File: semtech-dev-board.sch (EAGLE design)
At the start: 62 parts, among them Q1 BSS123, Q2 32MHz, U1 SEMTECH_SX1236, U2 QUALCOMM-TDK_B3588, U3 MIC5219 3.3V, U4 QUALCOMM-TDK_B3710

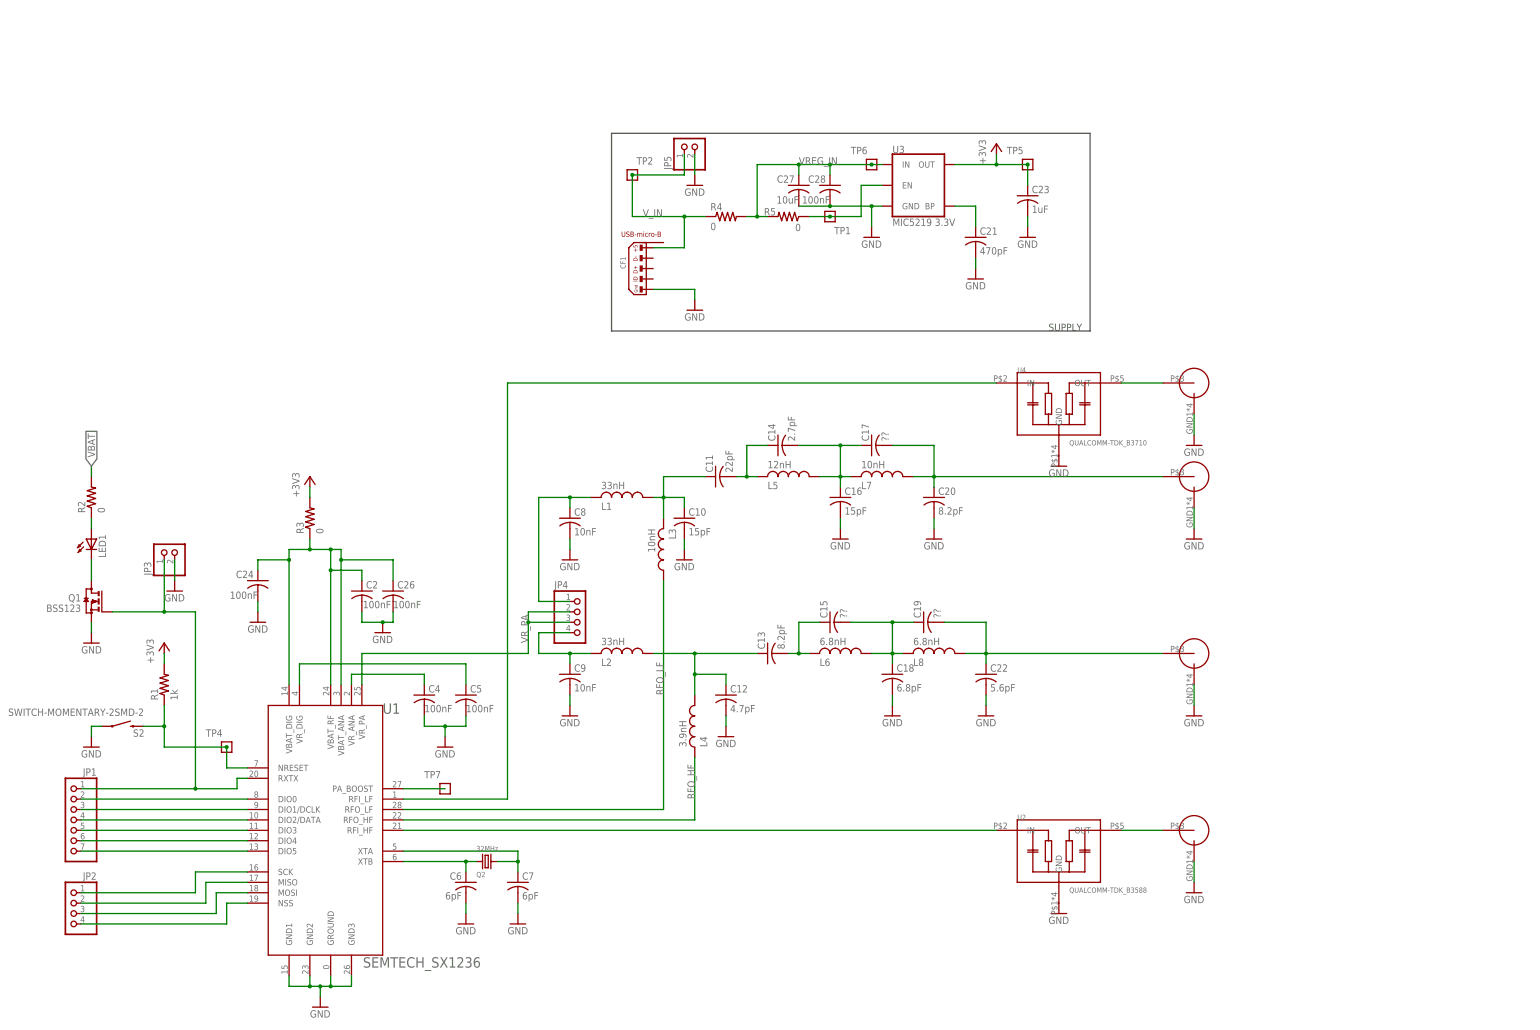
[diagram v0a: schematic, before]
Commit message: Tuesday D/R
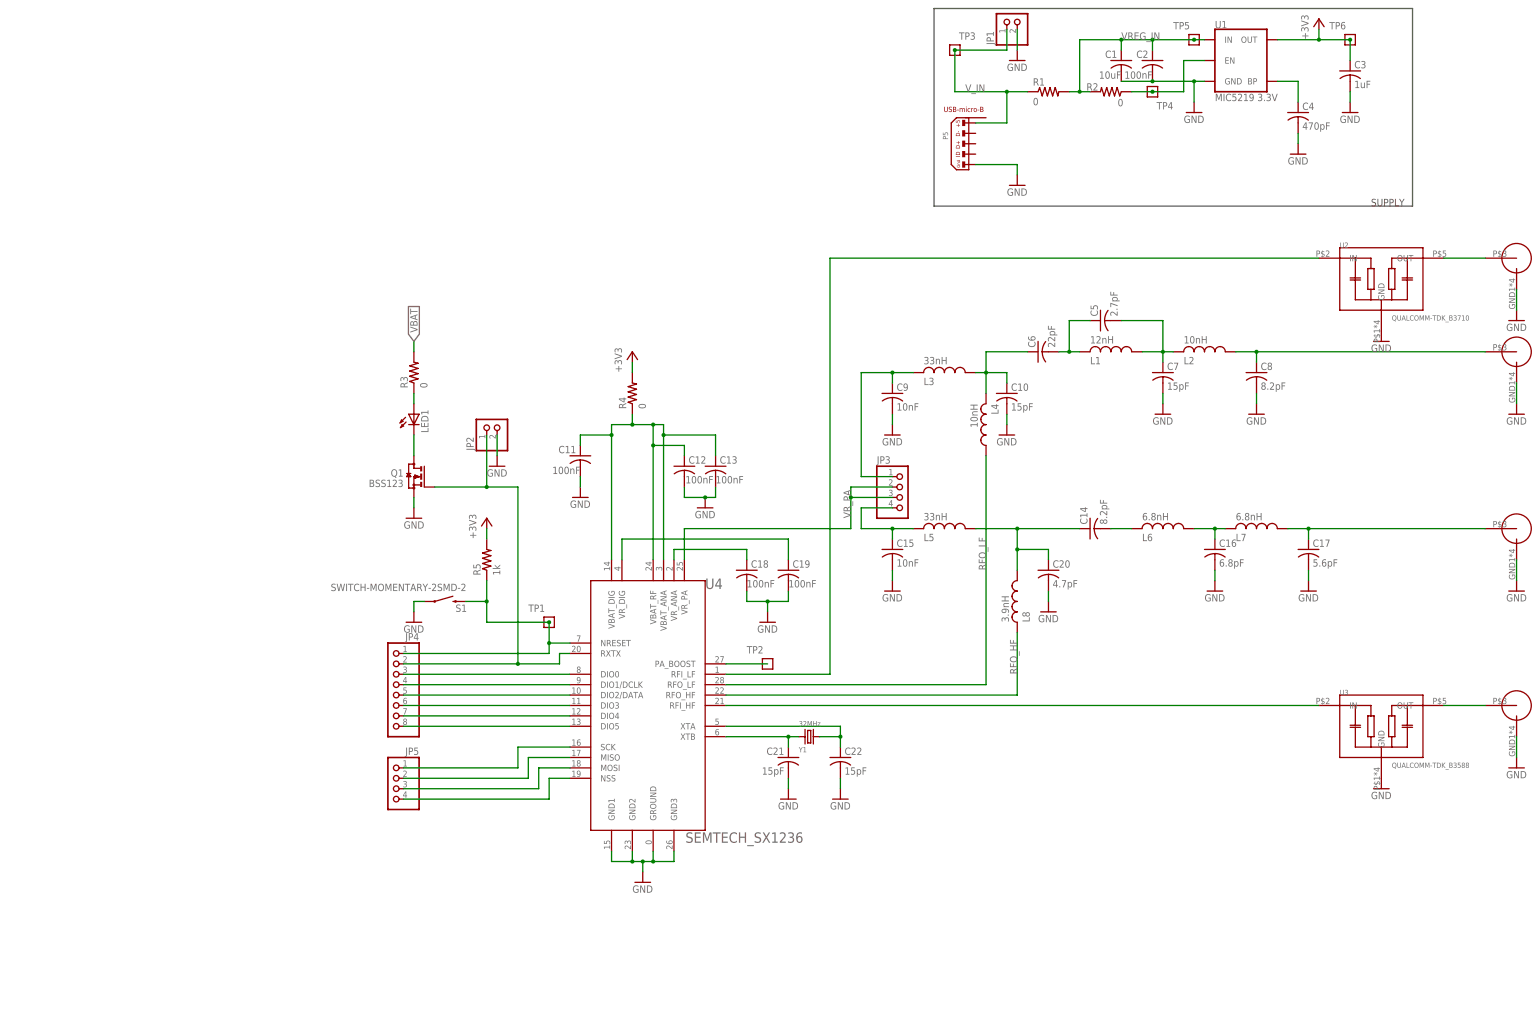
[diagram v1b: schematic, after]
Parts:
- removed C23: 1uF, rcl:C-USC0805
- removed C24, C26, C28: 100nF, rcl:C-USC0805
- removed C27: 10uF, rcl:C-USC0805
- removed CF1: (no value), psas_c3_team05:CON_USB-MICRO-B-RECEPTACLE-PTH-HIROSE-ZX62D-B-5P8
- removed Q2: 32MHz, low-gain-radio:CRYSTAL2.5X2.0MM
- removed S2: SWITCH-MOMENTARY-2SMD-2, psas_c3_team05:SWITCH-MOMENTARY-2SMD-2
- removed TP7: TEST-POINT, low-gain-radio:TEST-POINT
- removed U$1, U$2, U$3, U$4: SMAJ716-ND, psas_c3_team05:SMAJ716-ND
- added C1: 10uF, rcl:C-USC0805
- added C3: 1uF, rcl:C-USC0805
- added P1, P2, P3, P4: SMAJ716-ND, psas_c3_team05:SMAJ716-ND
- added P5: (no value), psas_c3_team05:CON_USB-MICRO-B-RECEPTACLE-PTH-HIROSE-ZX62D-B-5P8
- added S1: SWITCH-MOMENTARY-2SMD-2, psas_c3_team05:SWITCH-MOMENTARY-2SMD-2
- added TP3: TEST-POINT, low-gain-radio:TEST-POINT
- added Y1: 32MHz, low-gain-radio:CRYSTAL2.5X2.0MM
- C11: value 22pF -> 100nF
- C12: value 4.7pF -> 100nF
- C13: value 8.2pF -> 100nF
- C14: value 2.7pF -> 8.2pF
- C15: value ?? -> 10nF
- C16: value 15pF -> 6.8pF
- C17: value ?? -> 5.6pF
- C18: value 6.8pF -> 100nF
- C19: value ?? -> 100nF
- C20: value 8.2pF -> 4.7pF
- C21: value 470pF -> 15pF
- C22: value 5.6pF -> 15pF
- C4: value 100nF -> 470pF
- C5: value 100nF -> 2.7pF
- C6: value 6pF -> 22pF
- C7: value 6pF -> 15pF
- C8: value 10nF -> 8.2pF
- JP1: device pinhead:PINHD-1X7 -> pinhead:PINHD-1X2
- JP2: device pinhead:PINHD-1X4 -> pinhead:PINHD-1X2
- JP3, JP5: device pinhead:PINHD-1X2 -> pinhead:PINHD-1X4
- JP4: device pinhead:PINHD-1X4 -> pinhead:PINHD-1X8
- L1: value 33nH -> 12nH; device rcl:L-USL3230M -> rcl:L-USL3225M
- L2: value 33nH -> 10nH; device rcl:L-USL3230M -> rcl:L-USL3225M
- L3: value 10nH -> 33nH; device rcl:L-USL3230M -> rcl:L-USL3225M
- L4: value 3.9nH -> 10nH; device rcl:L-USL3230M -> rcl:L-USL3225P
- L5: value 12nH -> 33nH; device rcl:L-USL1812 -> rcl:L-USL3225P
- L6: device rcl:L-USL3230M -> rcl:L-USL3225M
- L7: value 10nH -> 6.8nH; device rcl:L-USL3230M -> rcl:L-USL3225M
- L8: value 6.8nH -> 3.9nH; device rcl:L-USL3230M -> rcl:L-USL3225M
- R1: value 1k -> 0
- R5: value 0 -> 1k
- U1: value SEMTECH_SX1236 -> MIC5219 3.3V; device low-gain-radio:SEMTECH_SX1236 -> SparkFun-IC-Power:V_REG_MIC52193.3V
- U2: value QUALCOMM-TDK_B3588 -> QUALCOMM-TDK_B3710; device low-gain-radio:QUALCOMM-TDK_B3588 -> low-gain-radio:QUALCOMM-TDK_B3710
- U3: value MIC5219 3.3V -> QUALCOMM-TDK_B3588; device SparkFun-IC-Power:V_REG_MIC52193.3V -> low-gain-radio:QUALCOMM-TDK_B3588
- U4: value QUALCOMM-TDK_B3710 -> SEMTECH_SX1236; device low-gain-radio:QUALCOMM-TDK_B3710 -> low-gain-radio:SEMTECH_SX1236
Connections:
- removed net DIO0: JP1.2, U1.DIO0
- removed net DIO1: JP1.3, U1.DIO1/DCLK
- removed net DIO2: JP1.4, U1.DIO2/DATA
- removed net DIO3: JP1.5, U1.DIO3
- removed net DIO4: JP1.6, U1.DIO4
- removed net DIO5: JP1.7, U1.DIO5
- new net N$2: JP4.8, U4.DIO5
- new net N$4: JP4.7, U4.DIO4
- new net N$6: JP4.6, U4.DIO3
- new net N$7: JP4.5, U4.DIO2/DATA
- new net N$8: JP4.4, U4.DIO1/DCLK
- new net N$9: JP4.3, U4.DIO0
- net +3V3: now also C3.1, R4.2, R5.2, TP6.1, U1.OUT; no longer C23.1, R1.2, R3.2, TP5.1, U3.OUT
- net BP: now also C4.1, U1.BP; no longer C21.1, U3.BP
- net GND: now also C1.2, C11.2, C13.2, C15.2, C17.2, C19.2, C3.2, JP1.2, JP2.2, P1.OUTERCONDUCTOR, P2.OUTERCONDUCTOR, P3.OUTERCONDUCTOR, P4.OUTERCONDUCTOR, P5.5, S1.1, U1.GND, U4.GND1, U4.GND2, U4.GND3, U4.GROUND; no longer C23.2, C24.2, C26.2, C27.2, C28.2, C5.2, C6.2, CF1.5, JP3.2, JP5.2, S2.1, U$1.OUTERCONDUCTOR, U$2.OUTERCONDUCTOR, U$3.OUTERCONDUCTOR, U$4.OUTERCONDUCTOR, U1.GND1, U1.GND2, U1.GND3, U1.GROUND, U4.GND
- net HFO_PA_HEAD: now also C15.1, JP3.4, L5.2; no longer C9.1, JP4.4, L2.2
- net LED+: now also R3.1; no longer R2.1
- net LFO_PA_HEAD: now also C9.1, JP3.1, L3.2; no longer C8.1, JP4.1, L1.2
- net N$1: now also R2.1, TP4.1, U1.EN; no longer R5.1, TP1.1, U3.EN
- net N$5: now also P1.CENTERCONDUCTOR, U2.OUT; no longer U$1.CENTERCONDUCTOR, U4.OUT
- net PA_BOOST: now also TP2.1, U4.PA_BOOST; no longer TP7.1, U1.PA_BOOST
- net RFI_HF: now also U3.IN, U4.RFI_HF; no longer U1.RFI_HF, U2.IN
- net RFI_HF_ANT: now also P4.CENTERCONDUCTOR, U3.OUT; no longer U$4.CENTERCONDUCTOR, U2.OUT
- net RFI_LF: now also U2.IN, U4.RFI_LF; no longer U1.RFI_LF, U4.IN
- net RFO_HF: now also L8.2, U4.RFO_HF; no longer L4.2, U1.RFO_HF
- net RFO_HF_1: now also C14.2; no longer C13.2, C15.1
- net RFO_HF_2: now also C16.1, L7.2; no longer C15.2, C18.1, C19.1, L8.2
- net RFO_HF_OUT: now also C17.1, L7.1, P3.CENTERCONDUCTOR; no longer C19.2, C22.1, L8.1, U$3.CENTERCONDUCTOR
- net RFO_HF_PA: now also C14.1, C20.1, L5.1, L8.1; no longer C12.1, C13.1, L2.1, L4.1
- net RFO_LF: now also L4.1, U4.RFO_LF; no longer L3.1, U1.RFO_LF
- net RFO_LF_1: now also C5.1, C6.2, L1.2; no longer C11.2, C14.1, L5.2
- net RFO_LF_2: now also C5.2, C7.1, L1.1, L2.2; no longer C14.2, C16.1, C17.1, L5.1, L7.2
- net RFO_LF_OUT: now also C8.1, L2.1, P2.CENTERCONDUCTOR; no longer C17.2, C20.1, L7.1, U$2.CENTERCONDUCTOR
- net RFO_LF_PA: now also C6.1, L3.1, L4.2; no longer C11.1, L1.1, L3.2
- net RXTX: now also JP2.1, JP4.2, U4.RXTX; no longer JP1.1, JP3.1, U1.RXTX
- net SPI_MISO: now also JP5.2, U4.MISO; no longer JP2.2, U1.MISO
- net SPI_MOSI: now also JP5.3, U4.MOSI; no longer JP2.3, U1.MOSI
- net SPI_NSS: now also JP5.4, U4.NSS; no longer JP2.4, U1.NSS
- net SPI_SCK: now also JP5.1, U4.SCK; no longer JP2.1, U1.SCK
- net SX1236_RST: now also JP4.1, R5.1, S1.2, TP1.1, U4.NRESET; no longer R1.1, S2.2, TP4.1, U1.NRESET
- net VBAT: now also C11.1, C12.1, C13.1, R3.2, R4.1, U4.VBAT_ANA, U4.VBAT_DIG, U4.VBAT_RF; no longer C2.1, C24.1, C26.1, R2.2, R3.1, U1.VBAT_ANA, U1.VBAT_DIG, U1.VBAT_RF
- net VREG_IN: now also C1.1, C2.1, R1.2, R2.2, TP5.1, U1.IN; no longer C27.1, C28.1, R4.2, R5.2, TP6.1, U3.IN
- net VR_ANA: now also C18.1, U4.VR_ANA; no longer C4.1, U1.VR_ANA
- net VR_DIG: now also C19.1, U4.VR_DIG; no longer C5.1, U1.VR_DIG
- net VR_PA: now also JP3.2, JP3.3, U4.VR_PA; no longer JP4.2, JP4.3, U1.VR_PA
- net V_IN: now also JP1.1, P5.1, R1.1, TP3.1; no longer CF1.1, JP5.1, R4.1, TP2.1
- net XTALA: now also C22.1, U4.XTA, Y1.2; no longer C7.1, Q2.2, U1.XTA
- net XTALB: now also C21.1, U4.XTB, Y1.1; no longer C6.1, Q2.1, U1.XTB
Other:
- moved on the sheet: C10, C11, C12, C13, C14, C15, C16, C17, C18, C19, C2, C20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
